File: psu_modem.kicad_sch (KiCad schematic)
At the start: 9 parts, among them U10 LM2596S-ADJ

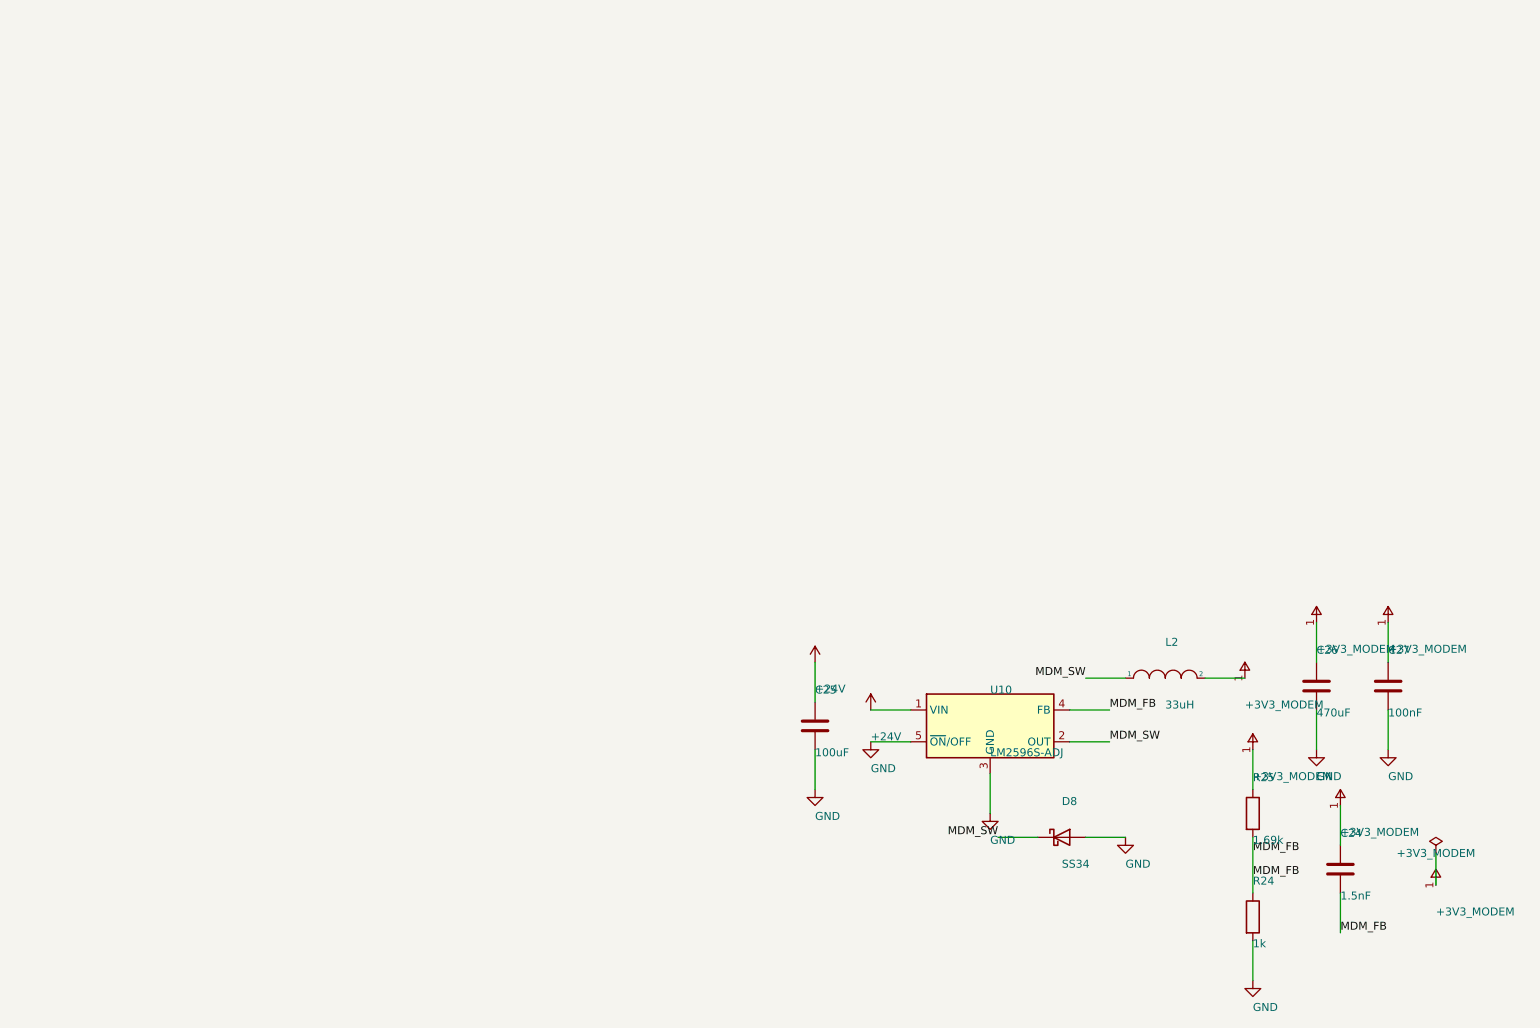
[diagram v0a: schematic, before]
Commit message: friday changes
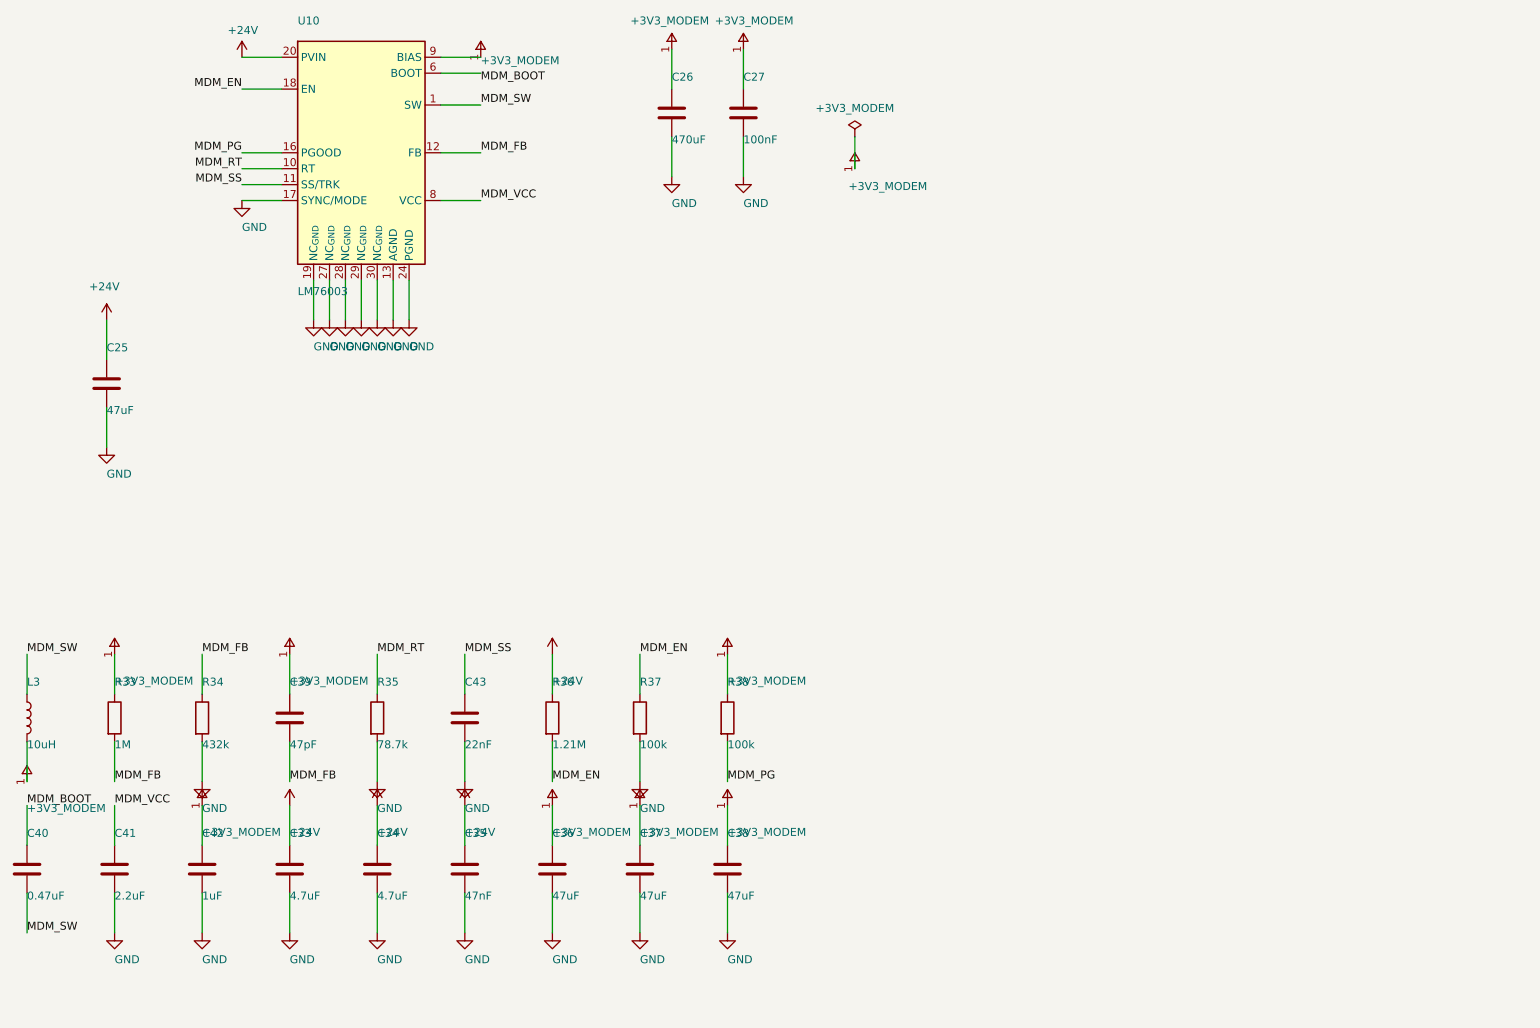
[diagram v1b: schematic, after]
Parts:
- removed C24: 1.5nF, Capacitor_SMD:C_0805_2012Metric_Pad1.18x1.45mm_HandSolder, symbol Device:C
- removed D8: SS34, Diode_SMD:D_SMA, symbol Device:D_Schottky
- removed L2: 33uH, Inductor_SMD:L_Bourns_SDR1806, symbol pspice:INDUCTOR
- removed R24: 1k, Resistor_SMD:R_1206_3216Metric_Pad1.30x1.75mm_HandSolder, symbol Device:R
- removed R25: 1.69k, Resistor_SMD:R_1206_3216Metric_Pad1.30x1.75mm_HandSolder, symbol Device:R
- removed U10: LM2596S-ADJ, Package_TO_SOT_SMD:TO-263-5_TabPin3, symbol Regulator_Switching:LM2596S-ADJ
- added C33, C34: 4.7uF, Capacitor_SMD:C_1210_3225Metric, symbol Device:C
- added C35: 47nF, Capacitor_SMD:C_0805_2012Metric, symbol Device:C
- added C36, C37, C38: 47uF, Capacitor_SMD:C_1210_3225Metric, symbol Device:C
- added C39: 47pF, Capacitor_SMD:C_0402_1005Metric, symbol Device:C
- added C40: 0.47uF, Capacitor_SMD:C_0603_1608Metric, symbol Device:C
- added C41: 2.2uF, Capacitor_SMD:C_0603_1608Metric, symbol Device:C
- added C42: 1uF, Capacitor_SMD:C_0603_1608Metric, symbol Device:C
- added C43: 22nF, Capacitor_SMD:C_0402_1005Metric, symbol Device:C
- added L3: 10uH, Inductor_SMD:L_Bourns_SRR1260, symbol Device:L
- added R33: 1M, Resistor_SMD:R_0402_1005Metric, symbol Device:R
- added R34: 432k, Resistor_SMD:R_0402_1005Metric, symbol Device:R
- added R35: 78.7k, Resistor_SMD:R_0402_1005Metric, symbol Device:R
- added R36: 1.21M, Resistor_SMD:R_0402_1005Metric, symbol Device:R
- added R37, R38: 100k, Resistor_SMD:R_0402_1005Metric, symbol Device:R
- added U10: LM76003, Package_DFN_QFN:Texas_RNP0030B_WQFN-30-1EP_4x6mm_P0.5mm_EP1.8x4.5mm_ThermalVias, symbol Regulator_Switching:LM76003
- C25: value 100uF -> 47uF; footprint Capacitor_SMD:CP_Elec_8x10.5 -> Capacitor_SMD:CP_Elec_6.3x7.7; DigiKey (none) -> 4713-CV2-1H470MF80-RTR-ND; MPN (none) -> CV2-1H470MF80-R; Manufacturer (none) -> Cal-Chip Electronics, Inc.
- C26: DigiKey (none) -> 1189-2097-2-ND; MPN (none) -> 25TLV470M10X10.5; Manufacturer (none) -> Rubycon
- C27: DigiKey (none) -> 1276-1003-2-ND; MPN (none) -> CL21B104KBCNNNC; Manufacturer (none) -> Samsung Electro-Mechanics
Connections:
- net +24V: now also C33.1, C34.1, C35.1, R36.1, U10.20 (PVIN), U10.21 (PVIN), U10.22 (PVIN)
- net +3V3_MODEM: now also C36.1, C37.1, C38.1, C39.1, C42.1, L3.2, R33.1, R38.1, U10.9 (BIAS)
- net GND: now also C33.2, C34.2, C35.2, C36.2, C37.2, C38.2, C41.2, C42.2, C43.2, R34.2, R35.2, R37.2, U10.13 (AGND), U10.14 (AGND), U10.15 (AGND), U10.17 (SYNC/MODE), U10.19 (NC_{GND}), U10.24 (PGND), U10.25 (PGND), U10.26 (PGND), U10.27 (NC_{GND}), U10.28 (NC_{GND}), U10.29 (NC_{GND}), U10.30 (NC_{GND}), U10.31 (AGND)
- net MDM_FB: now also C39.2, R33.2, R34.1, U10.12 (FB)
- net MDM_SW: now also C40.2, L3.1, U10.1 (SW), U10.2 (SW), U10.3 (SW), U10.4 (SW), U10.5 (SW)
- new net MDM_BOOT: C40.1, U10.6 (BOOT)
- new net MDM_EN: R36.2, R37.1, U10.18 (EN)
- new net MDM_PG: R38.2, U10.16 (PGOOD)
- new net MDM_RT: R35.1, U10.10 (RT)
- new net MDM_SS: C43.1, U10.11 (SS/TRK)
- new net MDM_VCC: C41.1, U10.8 (VCC)
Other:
- title: PSU MODEM 3V3 - Convertidor reductor LM2596S-ADJ (+24V -> +3V3_MODEM) -> PSU MODEM 3V3 - Convertidor reductor sincrono LM76003 (+24V -> +3V3_MODEM)
- moved on the sheet: C25, C26, C27
